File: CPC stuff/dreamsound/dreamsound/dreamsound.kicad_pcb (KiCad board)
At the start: 2 copper layers, 43.8 x 71.1 mm, 22 parts, among them J1 Conn_02x25_Odd_Even, J2 Conn_02x07_Odd_Even, J3 DB25_Female, U2 74LS138, U3 74LS32

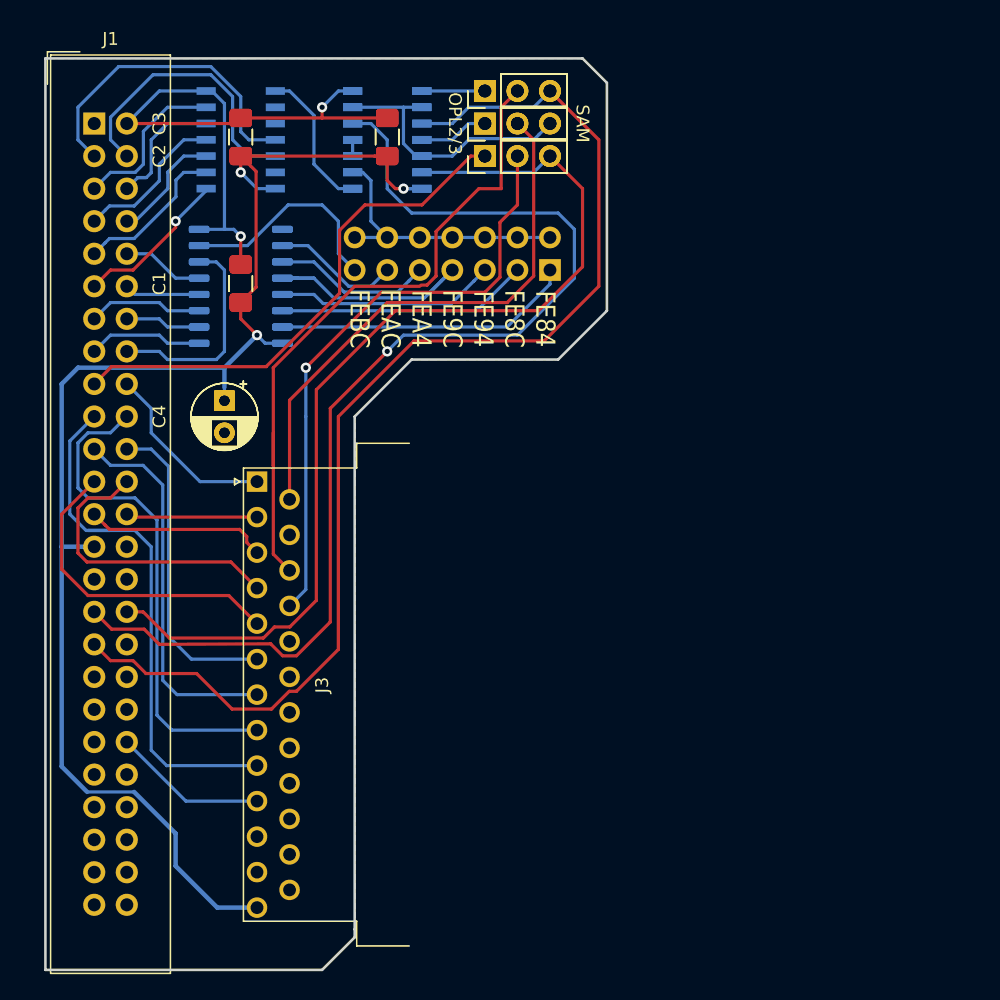
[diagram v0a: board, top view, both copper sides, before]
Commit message: Cleanups and improvements.
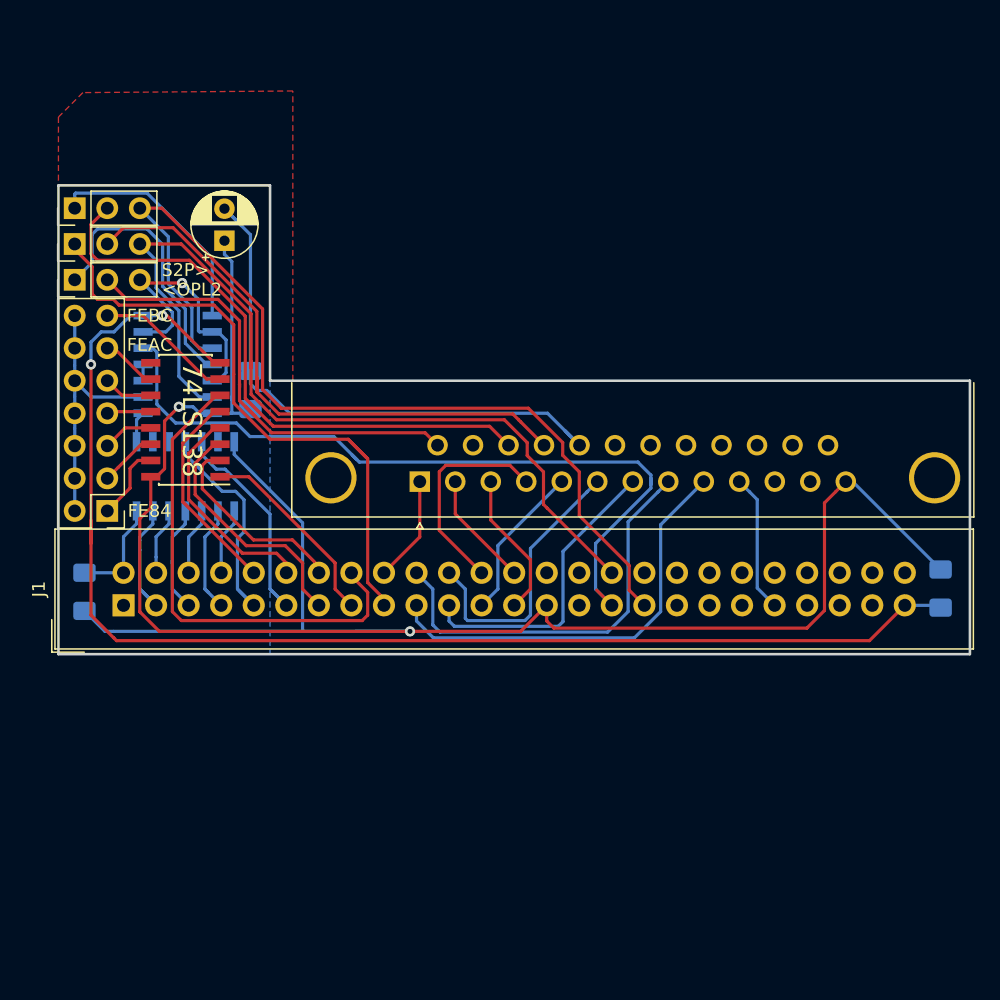
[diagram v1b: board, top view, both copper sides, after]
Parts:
- removed ? (x3): C, Capacitor_SMD:C_1206_3216Metric_Pad1.42x1.75mm_HandSolder
- removed ?: CP, Capacitor_THT:CP_Radial_D5.0mm_P2.50mm
- removed ?, OPL2/3, SAM: Jumper_3_Open, Connector_PinHeader_2.54mm:PinHeader_1x03_P2.54mm_Vertical
- removed LS138: 74LS138, Package_SO:SOIC-16_4.55x10.3mm_P1.27mm
- removed LS30: 74LS30, Package_SO:SOIC-14_3.9x8.7mm_P1.27mm
- removed LS32: 74LS32, Package_SO:SOIC-14_3.9x8.7mm_P1.27mm
- added U1: 74LS30, Package_SO:SOIC-14_3.9x8.7mm_P1.27mm, B.Cu at (24.9, 46.6)
- C1, C2, C3: moved to B.Cu
- J2: moved to F.Cu
- J3: footprint Connector_Dsub:DSUB-25_Female_Horizontal_P2.77x2.54mm_EdgePinOffset9.40mm -> Connector_Dsub:DSUB-25_Female_Horizontal_P2.77x2.84mm_EdgePinOffset4.94mm_Housed_MountingHolesOffset7.48mm
- U2: footprint Package_SO:SOIC-16_4.55x10.3mm_P1.27mm -> Package_SO:SOIC-16_3.9x9.9mm_P1.27mm; moved to F.Cu
- moved C3 65.0 mm to (83.8, 55.3), turned to 270 degrees
- moved C2 42.6 mm to (17.0, 55.6)
- moved J2 39.3 mm to (18.8, 49.3), turned to 180 degrees
- moved J1 37.7 mm to (20.1, 56.6), turned to 90 degrees
- moved JP2 34.2 mm to (16.3, 31.2)
- moved JP1 33.3 mm to (16.3, 25.7)
- moved JP3 32.7 mm to (16.3, 28.4)
- moved U3 24.0 mm to (24.3, 37.8)
- moved J3 12.7 mm to (43.2, 47.0), turned to 180 degrees
- moved C4 12.5 mm to (27.9, 28.2), turned to 90 degrees
- moved U2 11.3 mm to (24.9, 42.2), turned to 180 degrees
- moved C1 8.34 mm to (30.0, 39.8)
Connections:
- J1 pad 1: Net-(J1-Pad1) -> (no net)
- J1 pad 28: Net-(J1-Pad28) -> (no net)
- J1 pad 29: Net-(J1-Pad29) -> (no net)
- J1 pad 30: Net-(J1-Pad30) -> (no net)
- J1 pad 34: Net-(J1-Pad34) -> (no net)
- J1 pad 35: Net-(J1-Pad35) -> (no net)
- J1 pad 36: Net-(J1-Pad36) -> (no net)
- J1 pad 37: Net-(J1-Pad37) -> (no net)
- J1 pad 38: Net-(J1-Pad38) -> (no net)
- J1 pad 39: Net-(J1-Pad39) -> (no net)
- J1 pad 40: /!BUSRESET -> (no net)
- J1 pad 41: Net-(J1-Pad41) -> /!RESET
- J1 pad 42: Net-(J1-Pad42) -> (no net)
- J1 pad 43: Net-(J1-Pad43) -> (no net)
- J1 pad 44: Net-(J1-Pad44) -> (no net)
- J1 pad 45: Net-(J1-Pad45) -> (no net)
- J1 pad 46: Net-(J1-Pad46) -> (no net)
- J1 pad 47: Net-(J1-Pad47) -> (no net)
- J1 pad 48: Net-(J1-Pad48) -> (no net)
- J1 pad 50: Net-(J1-Pad50) -> (no net)
- J3 pad 10: /!BUSRESET -> /!RESET
- J3 pad 11: Net-(J3-Pad11) -> (no net)
- J3 pad 12: Net-(J3-Pad12) -> (no net)
- J3 pad 15: /IRQ -> (no net)
- U2 pad 9: Net-(U2-Pad9) -> (no net)
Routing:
- net GND: track 48.9 -> 157.7 mm
- net VCC: track 112.6 -> 163.1 mm, vias 3 -> 2
- net /!IORQ: track 87.6 -> 61.3 mm, vias 1 -> 0
- net /A2: track 16.7 -> 38.1 mm
- net /!WR: track 93.6 -> 73.4 mm
- net /FE9C-9F: track 21.1 -> 3.45 mm
- net /FE84-87: track 23.4 -> 5.93 mm
- net /A14: track 22.4 -> 5.25 mm
- net /!RDCS: track 5.45 -> 21.5 mm
- net /FE8C-8F: track 19.7 -> 4.50 mm
- net /A15: track 25.0 -> 9.99 mm
- net /!WRCS: track 4.92 -> 18.4 mm
- net /FE94-97: track 17.2 -> 3.97 mm
- net /D3: track 24.9 -> 12.2 mm
- net /!BUSRESET: track 12.1 -> 0.00 mm
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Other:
- board size 43.8 x 71.1 mm -> 71.1 x 36.6 mm
- net class Power added: clearance 0.2, trace_width 0.3302, via_dia 0.8, via_drill 0.4
- board text added: "74LS138"
- board text added: "74LS30"
- board text added: "74LS32"
- board text added: "<OPL2"
- board text added: "FE84"
- board text added: "FEAC"
- board text added: "FEBC"
- board text added: "S2P>"
- board text removed: "FE84 FE8C FE94 FE9C FEA4 FEAC FEBC"
